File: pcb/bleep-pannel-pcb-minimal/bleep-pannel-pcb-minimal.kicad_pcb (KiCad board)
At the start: 2 copper layers, 13.9 x 0.8 mm, 19 parts

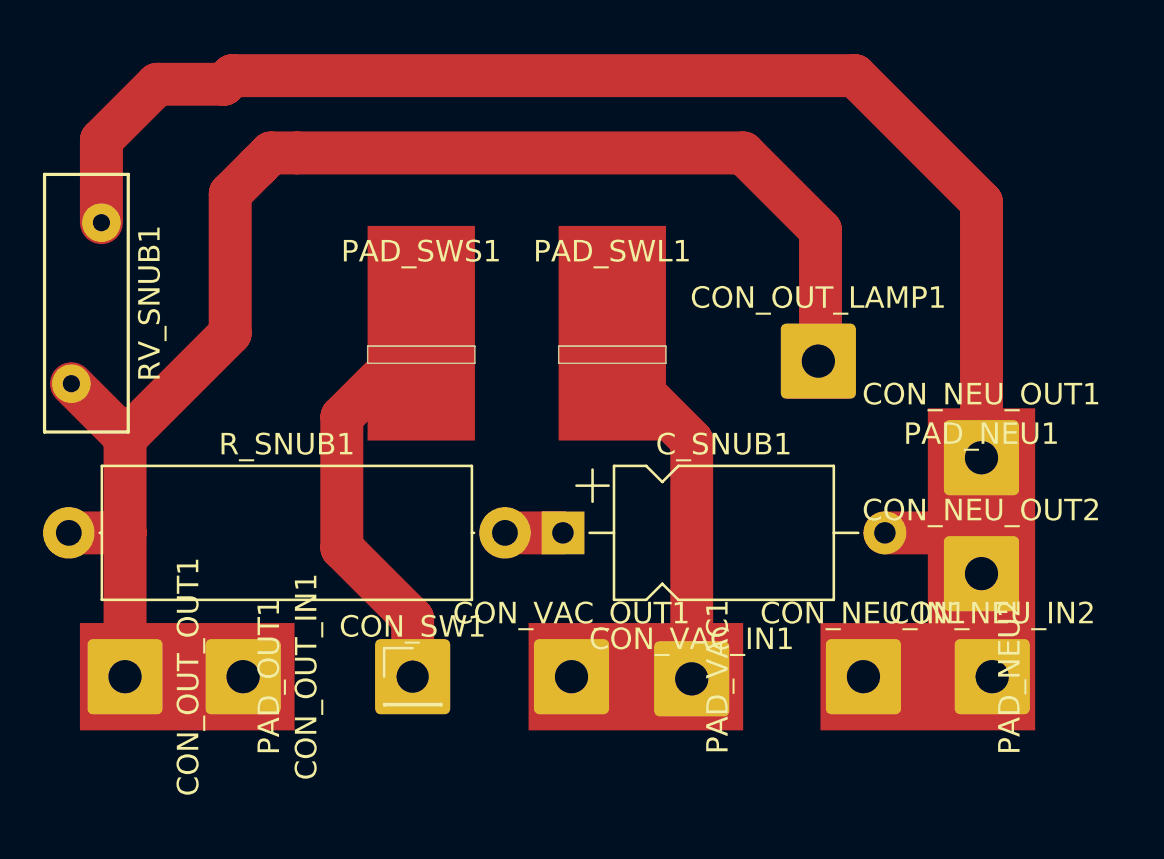
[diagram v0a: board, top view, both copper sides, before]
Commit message: A desk clamp and progress with minimal pannel
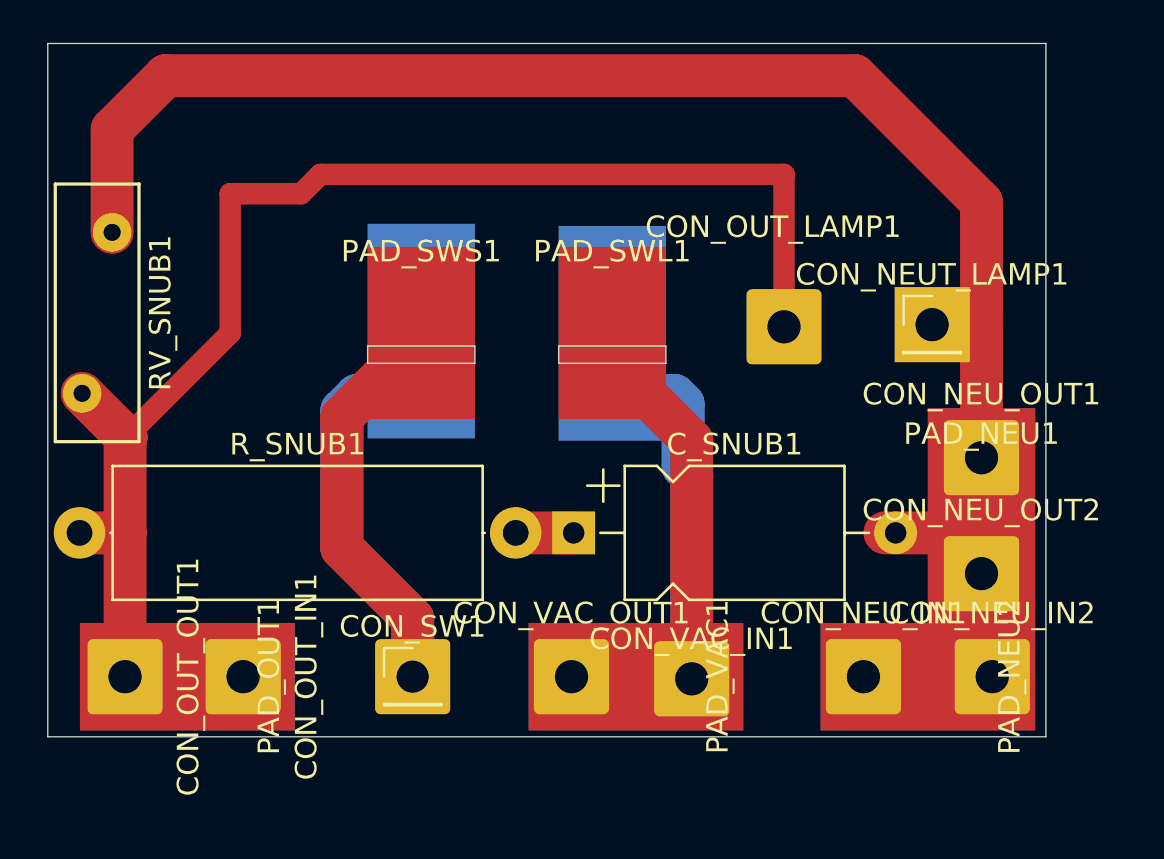
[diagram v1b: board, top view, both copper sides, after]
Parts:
- added ?: , , B.Cu at (6.00, 13.3)
- added ?: , , B.Cu at (14.9, 13.4)
- added CON_NEUT_LAMP1: Conn_01x01_Female, Connector_PinHeader_2.54mm:PinHeader_1x01_P2.54mm_Vertical, F.Cu at (29.8, 13.0)
- added PAD_NEU1: Conn_01x01_Female, Connector_Wire:SolderWirePad_1x01_SMD_5x10mm, B.Cu at (32.1, 21.9)
- added PAD_NEU2: Conn_01x01_Female, Connector_Wire:SolderWirePad_1x01_SMD_5x10mm, B.Cu at (29.6, 29.4)
- added PAD_OUT1: Conn_01x01_Female, Connector_Wire:SolderWirePad_1x01_SMD_5x10mm, B.Cu at (-4.90, 29.4)
- added PAD_VAC1: Conn_01x01_Female, Connector_Wire:SolderWirePad_1x01_SMD_5x10mm, B.Cu at (16.0, 29.4)
- moved CON_OUT_LAMP1 2.26 mm to (22.9, 13.1)
- moved RV_SNUB1 0.67 mm to (-9.80, 16.2)
- moved C_SNUB1 0.50 mm to (13.1, 22.7)
- moved R_SNUB1 0.50 mm to (-9.92, 22.7)
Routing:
- net Net-(CON_SW1-Pin_1): track 19.0 -> 36.7 mm
- net VAC: track 17.7 -> 34.1 mm
- net NEUT: track 68.0 -> 73.3 mm
- net Net-(CON_OUT_IN1-Pin_1): track 66.2 -> 62.9 mm
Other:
- board size 13.9 x 0.8 mm -> 46.5 x 32.3 mm
